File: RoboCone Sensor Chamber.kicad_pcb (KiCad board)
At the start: 2 copper layers, 85 x 43 mm, 47 parts, among them J1 Wurth 691210910002, J2 Wurth 691210910004, J3 Wurth 691210910004, J4 Wurth 691210910004, J5 Wurth 691210910004, J7 Wurth 691210910002, U1 ADS1234IPW, U2 TSR1-2450E, U3 TSR1-2433E

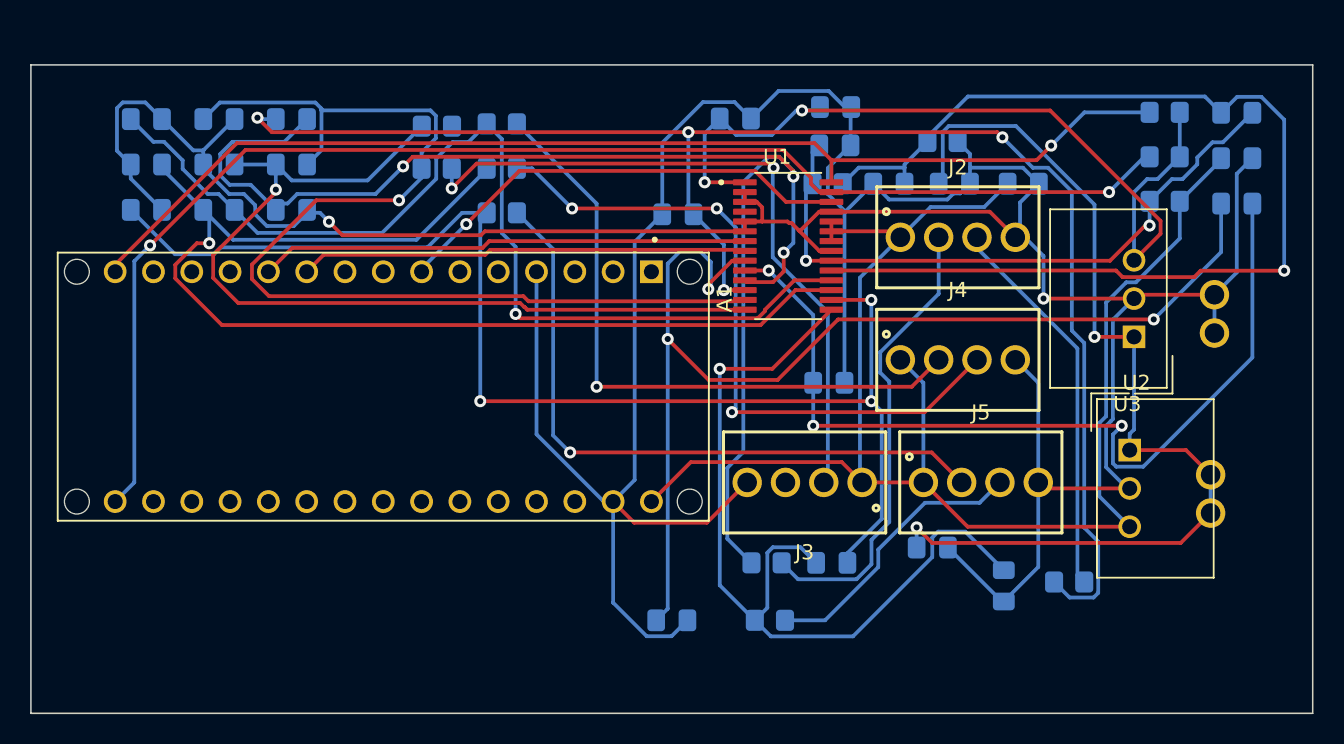
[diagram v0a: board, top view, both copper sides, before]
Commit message: lots of PCB changes
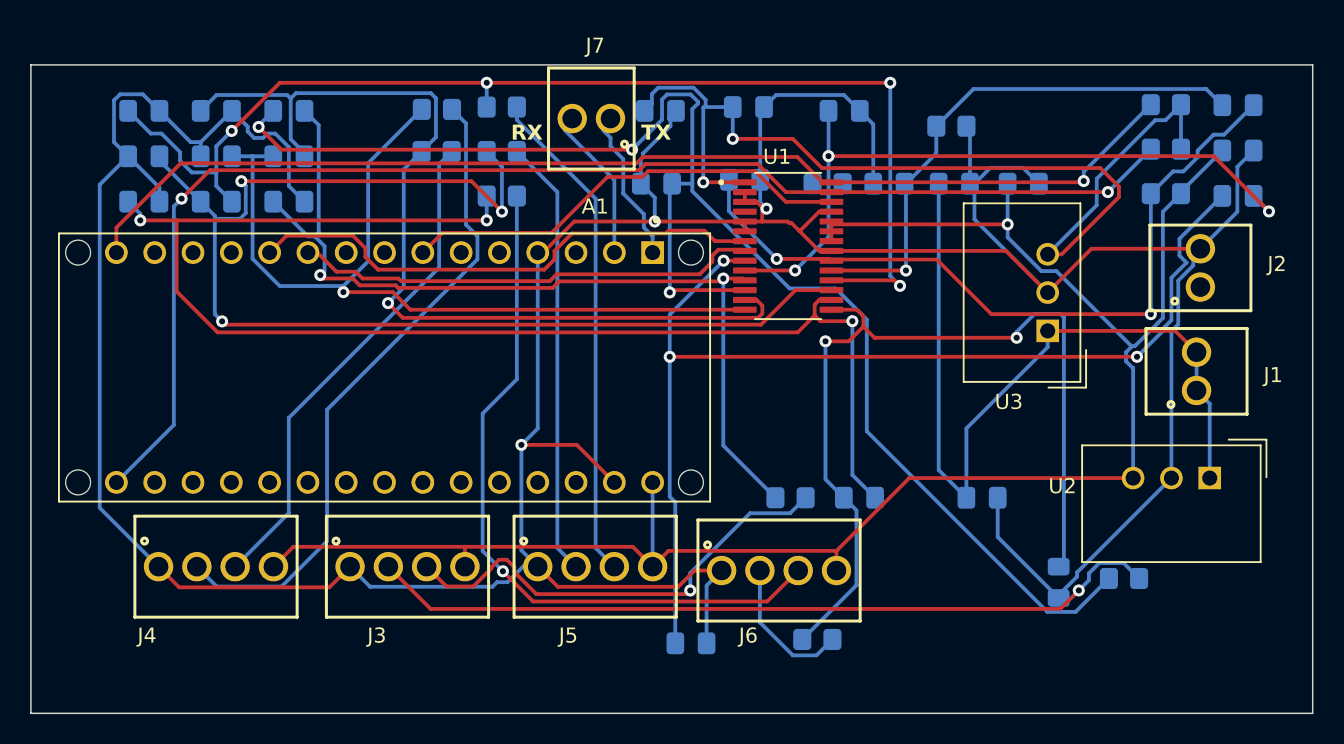
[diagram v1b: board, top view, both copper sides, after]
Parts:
- added J6: 691210910004, Robocone Footprints:691210910004, F.Cu at (152.9, 108.5)
- J1, J7: value Wurth 691210910002 -> 691210910002; moved to F.Cu
- J2: value Wurth 691210910004 -> 691210910002; footprint Robocone Footprints:691210910004 -> Robocone Footprints:691210910002
- J3, J4, J5: value Wurth 691210910004 -> 691210910004
- moved J4 51.1 mm to (115.6, 108.2)
- moved J7 43.3 mm to (140.5, 78.5), turned to 180 degrees
- moved J3 26.9 mm to (128.3, 108.2), turned to 0 degrees
- moved J5 26.2 mm to (140.7, 108.2)
- moved C23 18.1 mm to (157.2, 78.0)
- moved J2 16.2 mm to (180.8, 88.4), turned to 90 degrees
- moved J1 8.18 mm to (180.6, 95.2)
- moved C5 6.41 mm to (150.6, 82.5)
- moved C4 5.78 mm to (150.9, 77.7)
- moved U3 5.74 mm to (170.7, 92.6)
- moved U2 5.62 mm to (181.5, 102.3), turned to -90 degrees
- moved C9 5.00 mm to (145.0, 78.0)
- moved C17 4.69 mm to (158.2, 103.6)
- moved C22 4.67 mm to (166.4, 103.6)
- moved R6 4.60 mm to (153.7, 103.6)
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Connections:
- net Net-(C23-Pad2) renamed /CAPNET2
- net Net-(C24-Pad2) renamed /CAPNET1
- net Net-(U2-Vin) renamed /Input Power/V SUPPLY IN BOTH
- A1 pad 1: unconnected-(A1-D1/TX-Pad1) -> /TX1
- A1 pad 2: unconnected-(A1-D0/RX-Pad2) -> /RX1
- C1 pad 1: Net-(U1-REFP) -> /REFP1
- C1 pad 2: Net-(U1-REFN) -> /REFN1
- C5 pad 2: Net-(U1-REFP) -> /REFP1
- C6 pad 1: Net-(U1-REFN) -> /REFN1
- J2 pad 1: +5V -> unconnected-(J2-Pad1)
- J2 pad 2: /Load Cell Headers/AINP11 -> GND
- J3 pad 1: +5V -> GND
- J3 pad 2: Net-(J3-Pad2) -> /Load Cell Headers/AINN11
- J3 pad 3: unconnected-(J3-Pad3) -> /Load Cell Headers/AINP11
- J3 pad 4: GND -> +5V
- J4 pad 1: +5V -> GND
- J4 pad 2: Net-(J4-Pad2) -> /Load Cell Headers/AINN31
- J4 pad 3: Net-(J4-Pad3) -> /Load Cell Headers/AINP31
- J4 pad 4: GND -> +5V
- J5 pad 1: +5V -> GND
- J5 pad 2: Net-(J5-Pad2) -> /Load Cell Headers/AINN21
- J5 pad 3: Net-(J5-Pad3) -> /Load Cell Headers/AINP21
- J5 pad 4: GND -> +5V
- J7 pad 1: GND -> /TX1
- J7 pad 2: GND -> /RX1
- R10 pad 1: Net-(J4-Pad2) -> /Load Cell Headers/AINP21
- R11 pad 1: Net-(J4-Pad3) -> /Load Cell Headers/AINN21
- R12 pad 1: Net-(J5-Pad2) -> /Load Cell Headers/AINP41
- R13 pad 1: Net-(J5-Pad3) -> /Load Cell Headers/AINN41
- R3 pad 2: Net-(U1-REFP) -> /REFP1
- R4 pad 2: Net-(U1-REFN) -> /REFN1
- R8 pad 1: Net-(J3-Pad2) -> /Load Cell Headers/AINP31
- R9 pad 1: unconnected-(R9-Pad1) -> /Load Cell Headers/AINN31
- U1 pad 19: Net-(U1-REFN) -> /REFN1
- U1 pad 20: Net-(U1-REFP) -> /REFP1
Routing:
- net Net-(U1-REFN): track 74.9 -> 0.00 mm, vias 1 -> 0
- net /REFP1: track 0.00 -> 50.4 mm, vias 0 -> 2
- net /Load Cell Headers/AINP41: track 0.00 -> 47.6 mm, vias 0 -> 1
- net Net-(J4-Pad3): track 46.2 -> 0.00 mm, vias 3 -> 0
- net Net-(J3-Pad2): track 46.0 -> 0.00 mm, vias 2 -> 0
- net Net-(J5-Pad2): track 44.1 -> 0.00 mm, vias 1 -> 0
- net /Load Cell Headers/AINN31: track 0.00 -> 43.9 mm
- net Net-(J4-Pad2): track 43.0 -> 0.00 mm, vias 1 -> 0
- net Net-(U1-REFP): track 42.9 -> 0.00 mm, vias 2 -> 0
- net /REFN1: track 0.00 -> 35.9 mm, vias 0 -> 1
- net /Load Cell Headers/AINP31: track 0.00 -> 33.5 mm
- net /Load Cell Headers/AINP21: track 0.00 -> 33.2 mm
- net AINP1: track 90.0 -> 60.3 mm, vias 3 -> 2
- net /Load Cell Headers/AINN21: track 0.00 -> 29.2 mm
- net /Load Cell Headers/AINN11: track 25.8 -> 52.9 mm, vias 0 -> 1
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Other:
- board text added: "RX"
- board text added: "TX"
